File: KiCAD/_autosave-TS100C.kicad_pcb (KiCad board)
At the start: 4 copper layers, 84 x 10 mm, 63 parts, among them J1 USB_C_Receptacle_USB2.0, J2 OLED_64x32, J3 A, J4 B, J5 DNP, P1 TC2030-CTX, Q1 SS8050, Q2 DMP3017SFG, SW1 key1, SW2 key2, U1 USBLC6-4SC6, U2 AP2204R-3.3, U3 STUSB4500, U4 STM32F072C8Ux, U5 OPA340NA, U6 MCP9700AT-ETT, U7 SI8540

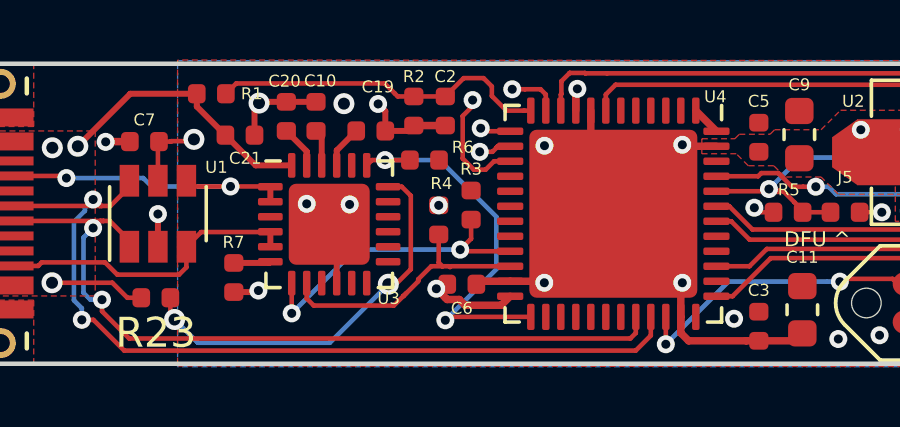
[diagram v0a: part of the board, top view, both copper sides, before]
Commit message: updated pcb
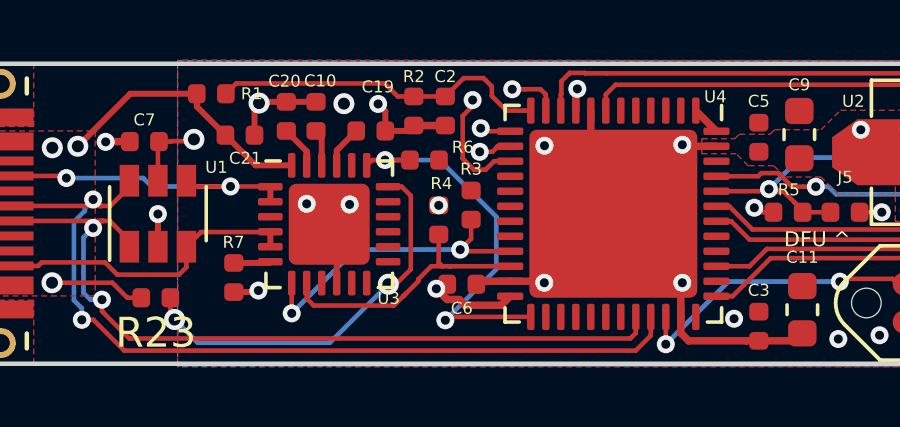
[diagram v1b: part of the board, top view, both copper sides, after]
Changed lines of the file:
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@@
     (thickness 1.6)
     (drawings 11)
-    (tracks 640)
+    (tracks 639)
     (zones 0)
     (modules 63)
@@
   (segment (start 102.35 86.75) (end 102.23 86.63) (width 0.154) (layer F.Cu) (net 11))
   (segment (start 102.580071 86.75) (end 102.35 86.75) (width 0.154) (layer F.Cu) (net 11))
-  (segment (start 102.606061 86.77599) (end 102.580071 86.75) (width 0.154) (layer F.Cu) (net 11))
   (segment (start 104.6125 86.75) (end 102.632051 86.75) (width 0.154) (layer F.Cu) (net 11))
-  (segment (start 102.632051 86.75) (end 102.606061 86.77599) (width 0.154) (layer F.Cu) (net 11))
   (segment (start 101.545998 87.184078) (end 101.545998 87.254002) (width 0.154) (layer F.Cu) (net 11))
   (segment (start 101.980076 86.75) (end 101.545998 87.184078) (width 0.154) (layer F.Cu) (net 11))
@@
   (segment (start 102.35 86.75) (end 101.980076 86.75) (width 0.154) (layer F.Cu) (net 11))
   (segment (start 101.053038 87.746962) (end 101.046962 87.746962) (width 0.154) (layer F.Cu) (net 11))
+  (segment (start 102.580071 86.75) (end 102.632051 86.75) (width 0.154) (layer F.Cu) (net 11))
   (via (at 97.33 88.32) (size 0.6) (drill 0.3) (layers F.Cu B.Cu) (net 12))
   (segment (start 97.33 87.3125) (end 97.33 88.32) (width 0.154) (layer F.Cu) (net 12))
